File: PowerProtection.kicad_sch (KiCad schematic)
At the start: 14 parts, among them U7 LM76202QPWPRQ1

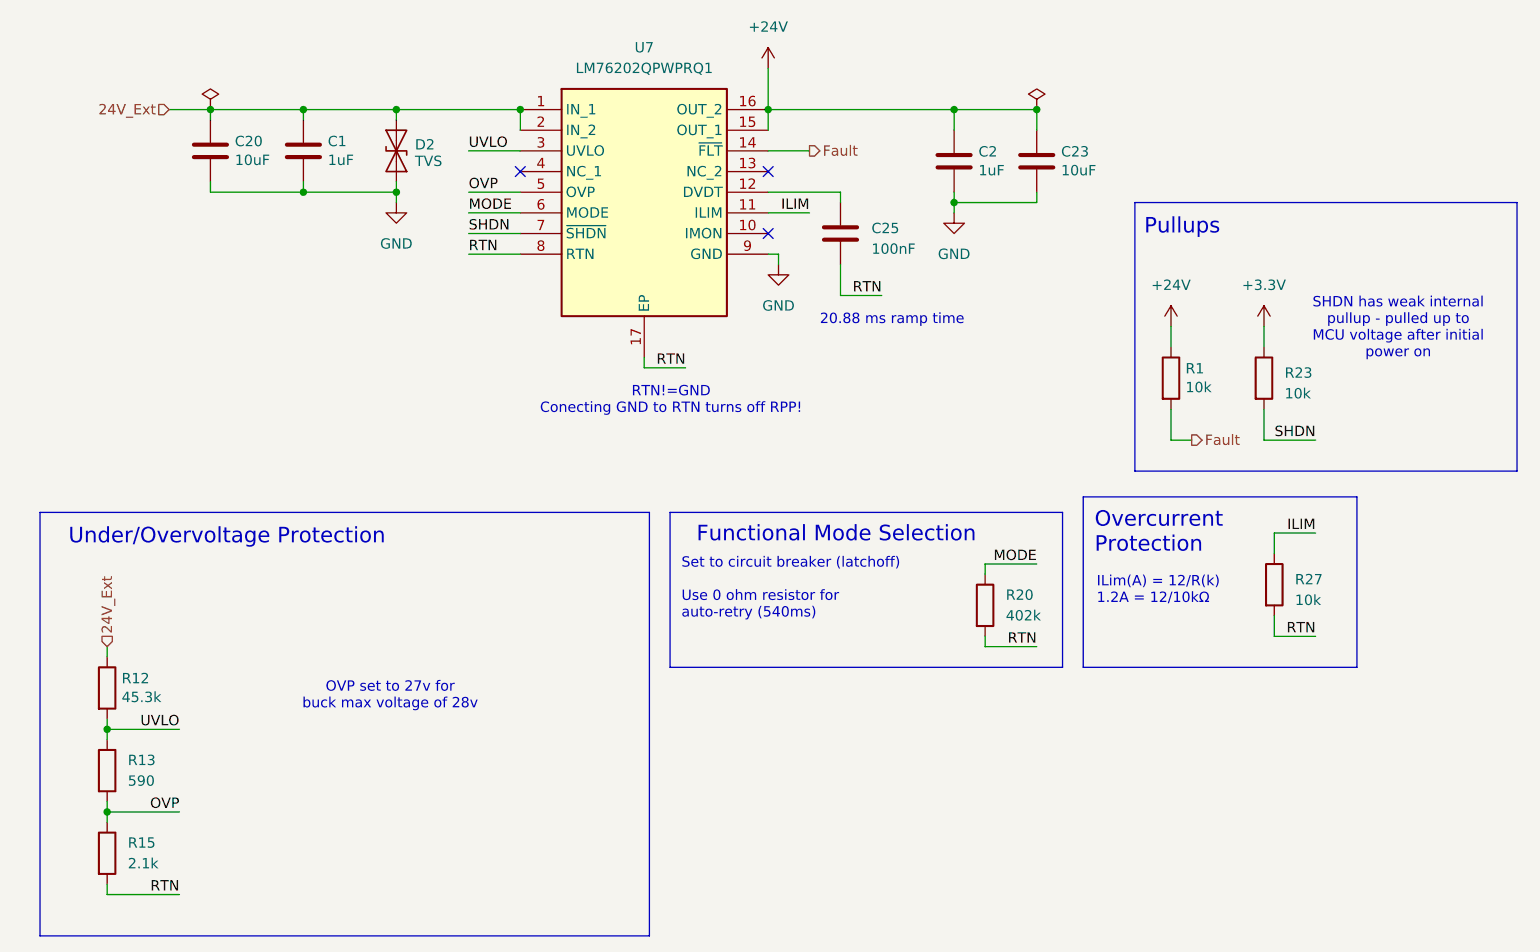
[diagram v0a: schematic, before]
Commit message: add IMON, change conn pinout
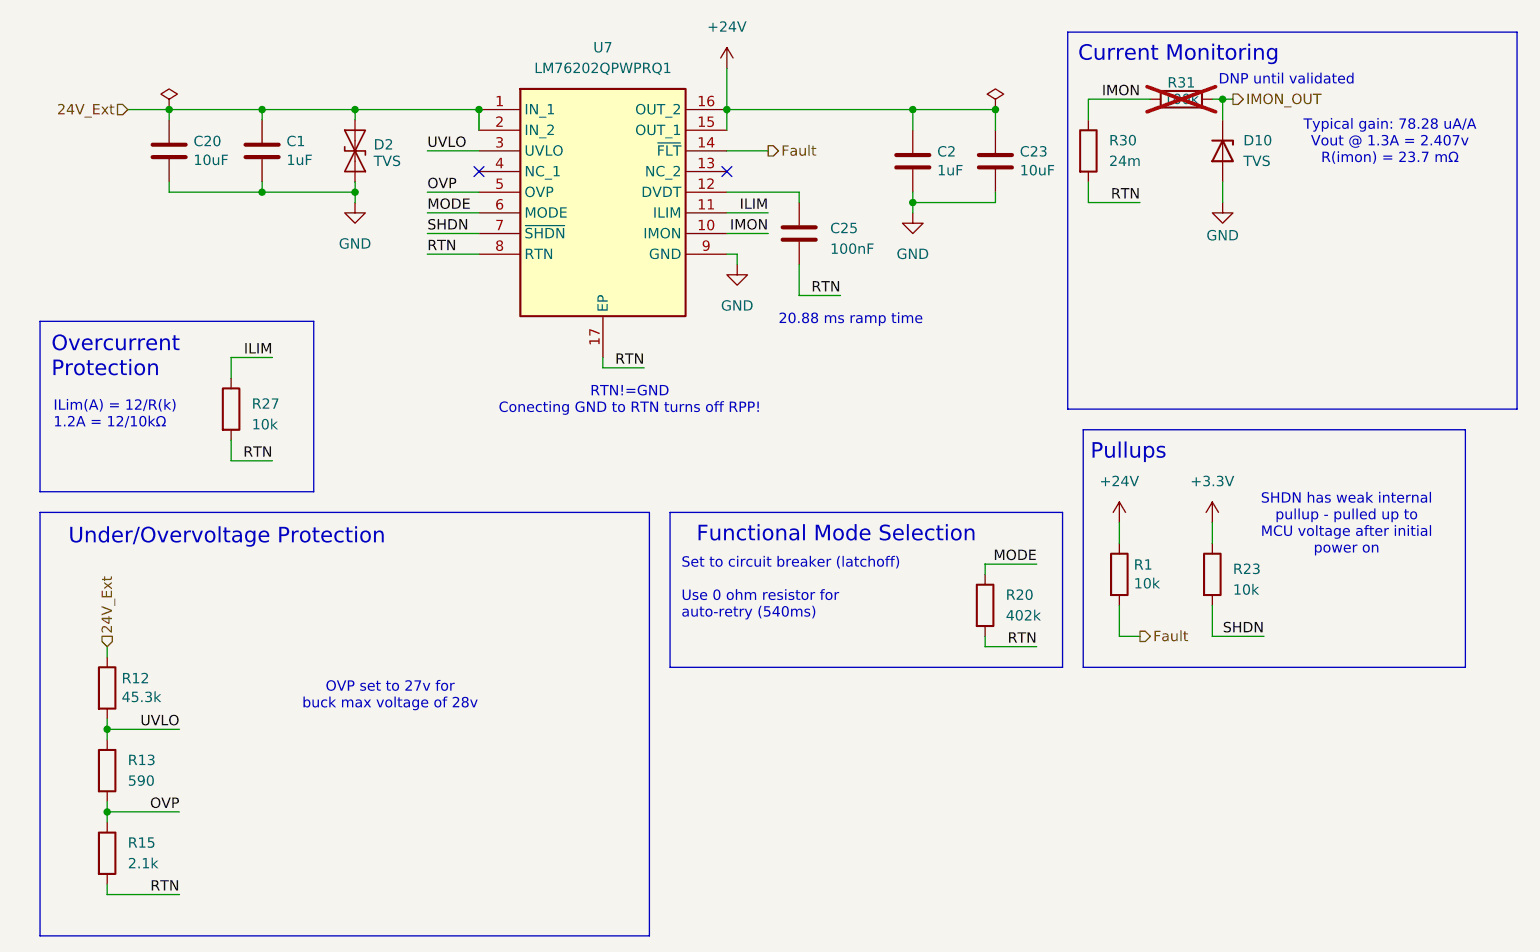
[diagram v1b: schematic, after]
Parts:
- added D10: TVS, symbol Device:D_Zener
- added R30: 24m, symbol Device:R
- added R31: 100k, symbol Device:R
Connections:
- net GND: now also D10.2 (A)
- net RTN: now also R30.2
- net IMON: now reaches U7.10 (IMON)
- net IMON: now also R30.1, R31.1
- new net IMON_OUT: D10.1 (K), R31.2
- no-connect marks 3 -> 2
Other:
- note added: "Current Monitoring"
- note added: "DNP until validated"
- note added: "Typical gain: 78.28 uA/A Vout @ 1.3A = 2.407v R(imon) = 23.7 mΩ"
- moved on the sheet: C1, C2, C20, C23, C25, D2, R1, R23, R27, U7

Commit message: add some footprints
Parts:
- R1, R12, R13, R15, R20, R23, R27, R30: footprint (none) -> Resistor_SMD:R_0603_1608Metric_Pad0.98x0.95mm_HandSolder
- R31: footprint (none) -> Resistor_SMD:R_0603_1608Metric_Pad0.98x0.95mm_HandSolder; P/N (none) -> CRCW0603100KFKEE
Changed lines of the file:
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@@
 			)
 		)
-		(property "Footprint" ""
+		(property "Footprint" "Resistor_SMD:R_0603_1608Metric_Pad0.98x0.95mm_HandSolder"
 			(at 153.67 32.258 90)
 			(effects
@@
 		(property "Description" "Resistor"
 			(at 153.67 30.48 0)
+			(effects
+				(font
+					(size 1.27 1.27)
+				)
+				(hide yes)
+			)
+		)
+		(property "P/N" "CRCW0603100KFKEE "
+			(at 153.67 30.48 90)
 			(effects
 				(font
@@
 			)
 		)
-		(property "Footprint" ""
+		(property "Footprint" "Resistor_SMD:R_0603_1608Metric_Pad0.98x0.95mm_HandSolder"
 			(at 127.762 92.71 90)
 			(effects
@@
 			)
 		)
-		(property "Footprint" ""
+		(property "Footprint" "Resistor_SMD:R_0603_1608Metric_Pad0.98x0.95mm_HandSolder"
 			(at 19.812 123.19 90)
 			(effects
@@
 			)
 		)
-		(property "Footprint" ""
+		(property "Footprint" "Resistor_SMD:R_0603_1608Metric_Pad0.98x0.95mm_HandSolder"
 			(at 144.272 88.9 90)
 			(effects
@@
 			)
 		)
-		(property "Footprint" ""
+		(property "Footprint" "Resistor_SMD:R_0603_1608Metric_Pad0.98x0.95mm_HandSolder"
 			(at 155.702 88.9 90)
 			(effects
@@
 			)
 		)
-		(property "Footprint" ""
+		(property "Footprint" "Resistor_SMD:R_0603_1608Metric_Pad0.98x0.95mm_HandSolder"
 			(at 35.052 68.58 90)
 			(effects
@@
 			)
 		)
-		(property "Footprint" ""
+		(property "Footprint" "Resistor_SMD:R_0603_1608Metric_Pad0.98x0.95mm_HandSolder"
 			(at 140.462 36.83 90)
 			(effects
@@
 			)
 		)
-		(property "Footprint" ""
+		(property "Footprint" "Resistor_SMD:R_0603_1608Metric_Pad0.98x0.95mm_HandSolder"
 			(at 19.812 113.03 90)
 			(effects
@@
 			)
 		)
-		(property "Footprint" ""
+		(property "Footprint" "Resistor_SMD:R_0603_1608Metric_Pad0.98x0.95mm_HandSolder"
 			(at 19.812 102.87 90)
 			(effects
